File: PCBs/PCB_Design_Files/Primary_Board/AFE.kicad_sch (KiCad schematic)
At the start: 25 parts, among them U1 OPA381, U2 TLV9002, U3 TLV9002, U4 TLV9002

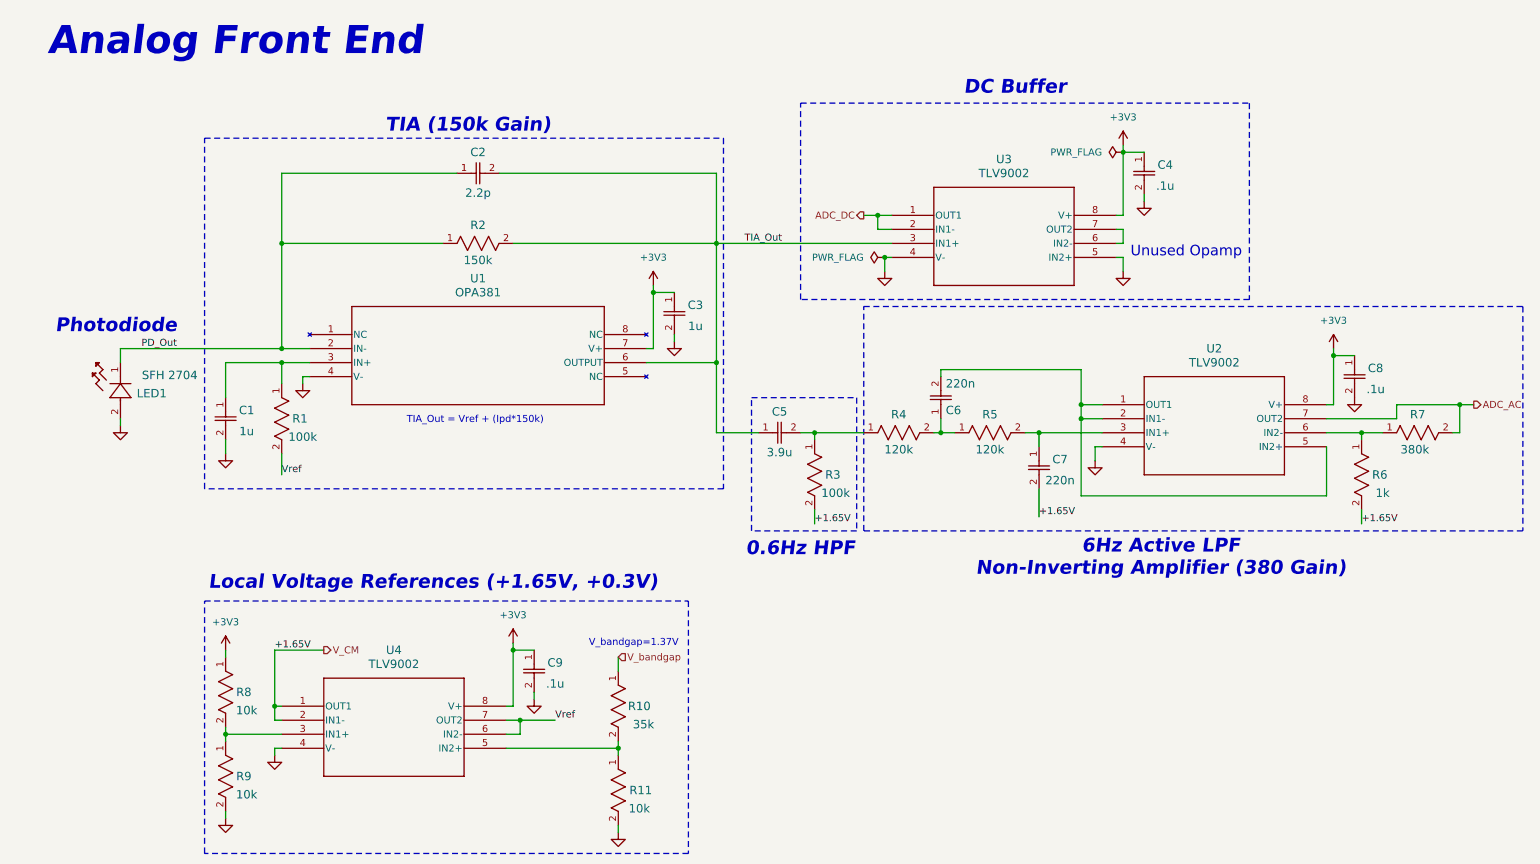
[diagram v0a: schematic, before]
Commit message: updated AFE pcb
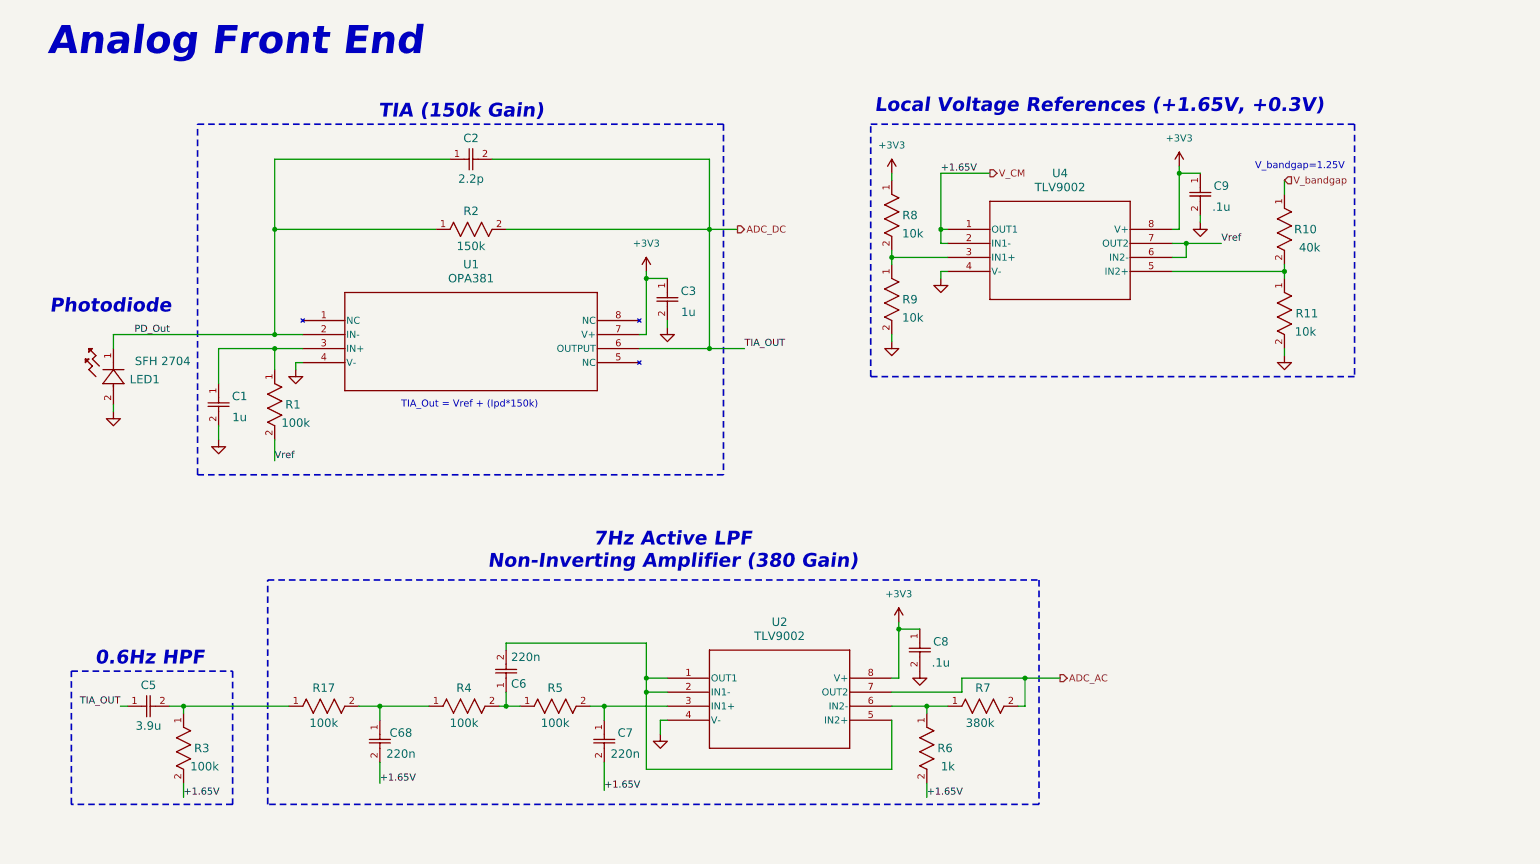
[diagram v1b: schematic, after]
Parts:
- removed C4: .1u, Project Footprints:0603_capacitor, symbol project_symbols:0603_capacitor
- removed U3: TLV9002, Project Footprints:TLV9002, symbol project_symbols:TLV9002
- added C68: 220n, Project Footprints:0603_capacitor, symbol project_symbols:0603_capacitor
- added R17: 100k, Project Footprints:0603_resistor, symbol project_symbols:0603_resistor
- R10: value 35k -> 40k
- R4, R5: value 120k -> 100k
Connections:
- net TIA_Out is gone; now on net ADC_DC: C2.2, C5.1, R2.2, U1.6 (OUTPUT)
- net V_CM: now also C68.2
- net at C5.2, R3.1: now also R17.1; no longer R4.1
- new net: C68.1, R17.2, R4.1
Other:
- note added: "7Hz Active LPF Non-Inverting Amplifier (380 Gain)"
- note added: "V_bandgap=1.25V"
- note removed: "6Hz Active LPF Non-Inverting Amplifier (380 Gain)"
- note removed: "DC Buffer"
- note removed: "Unused Opamp"
- note removed: "V_bandgap=1.37V"
- moved on the sheet: C1, C2, C3, C5, C6, C7, C8, C9, LED1, R1, R10, R11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
